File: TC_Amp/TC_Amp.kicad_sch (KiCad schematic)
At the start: 60 parts, among them J1 Screw_Terminal_01x02, J2 Screw_Terminal_01x02, J3 Conn_01x04_Pin, J4 Screw_Terminal_01x02, J5 Screw_Terminal_01x02, Q1 PMOS, U1 LT1025CN8-PBF, U10 LT1025CN8-PBF, U11 LM741, U12 LTC1049CN8_PBF, U13 LTC1049CN8_PBF, U14 LM317T, U2 LTC1049CN8_PBF, U3 LT1054, U4 LM741, U5 LTC1049CN8_PBF, U6 LT1025CN8-PBF, U7 LM741, U8 LTC1049CN8_PBF, U9 LTC1049CN8_PBF

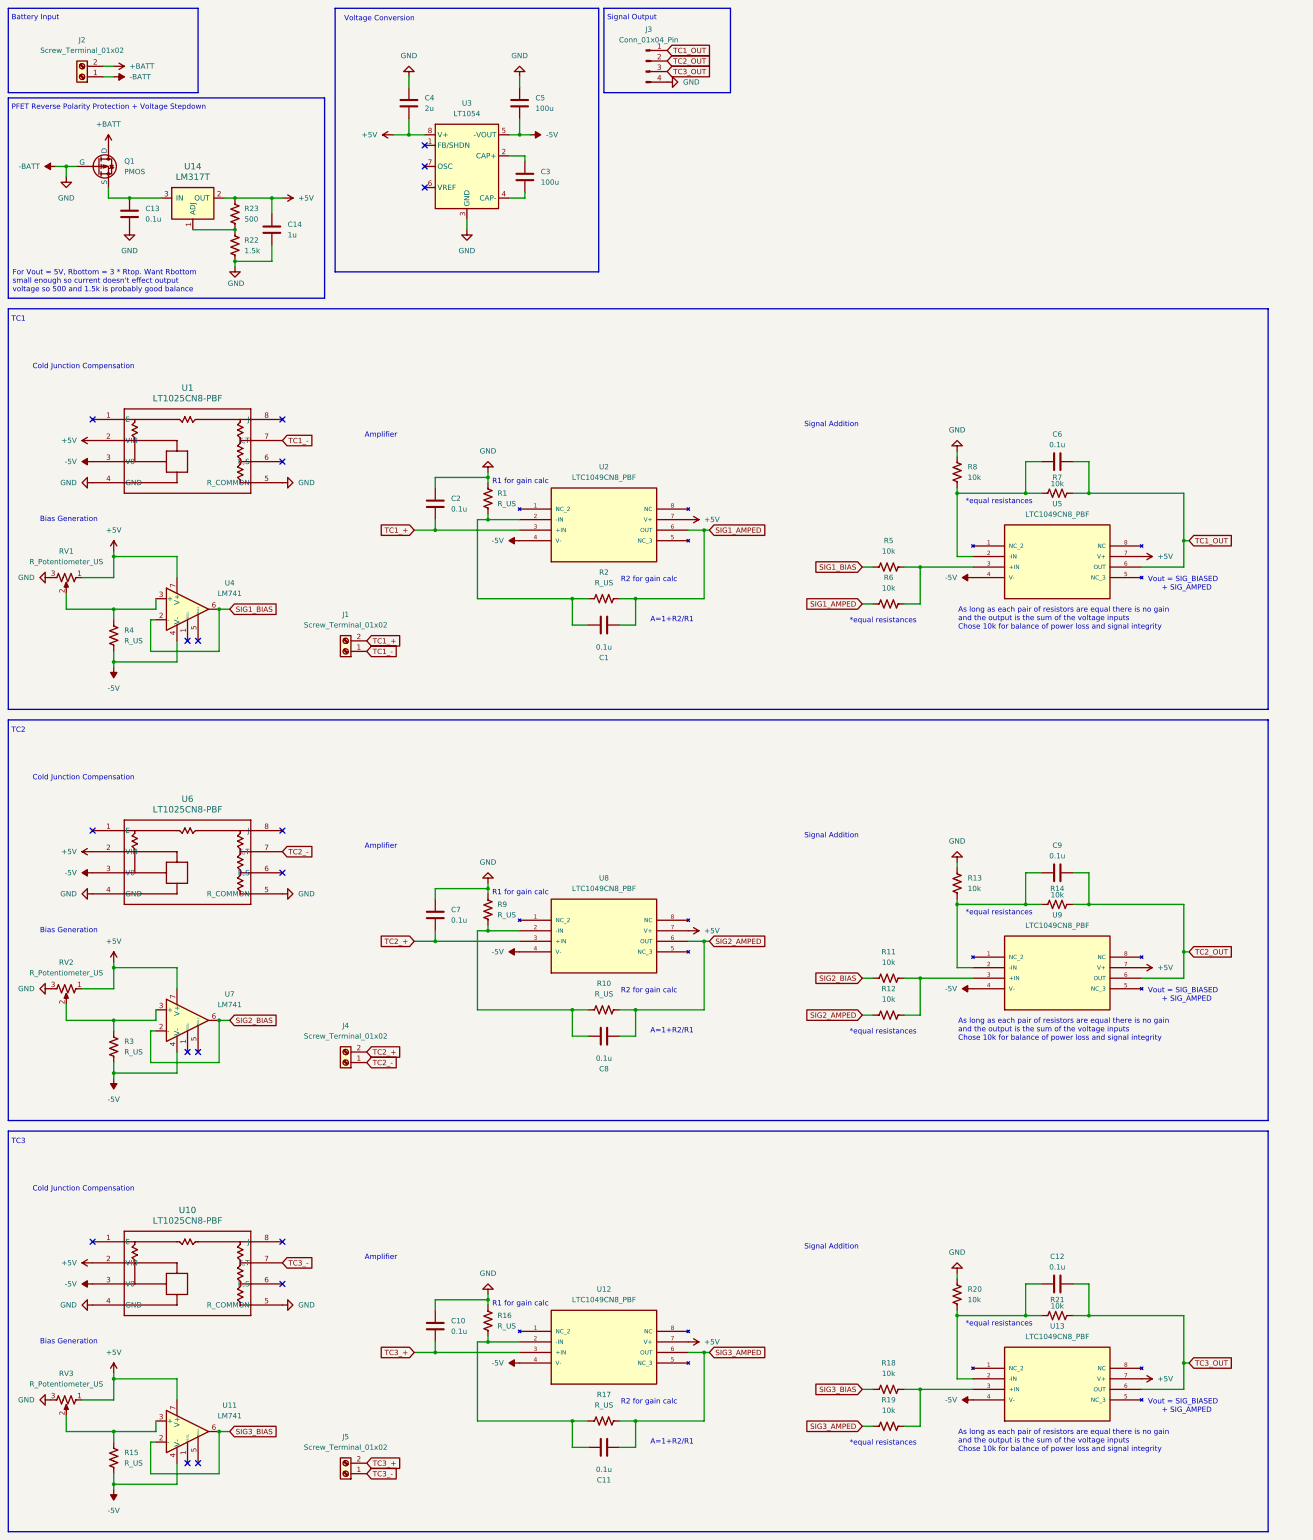
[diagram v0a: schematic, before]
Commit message: change to common cjc
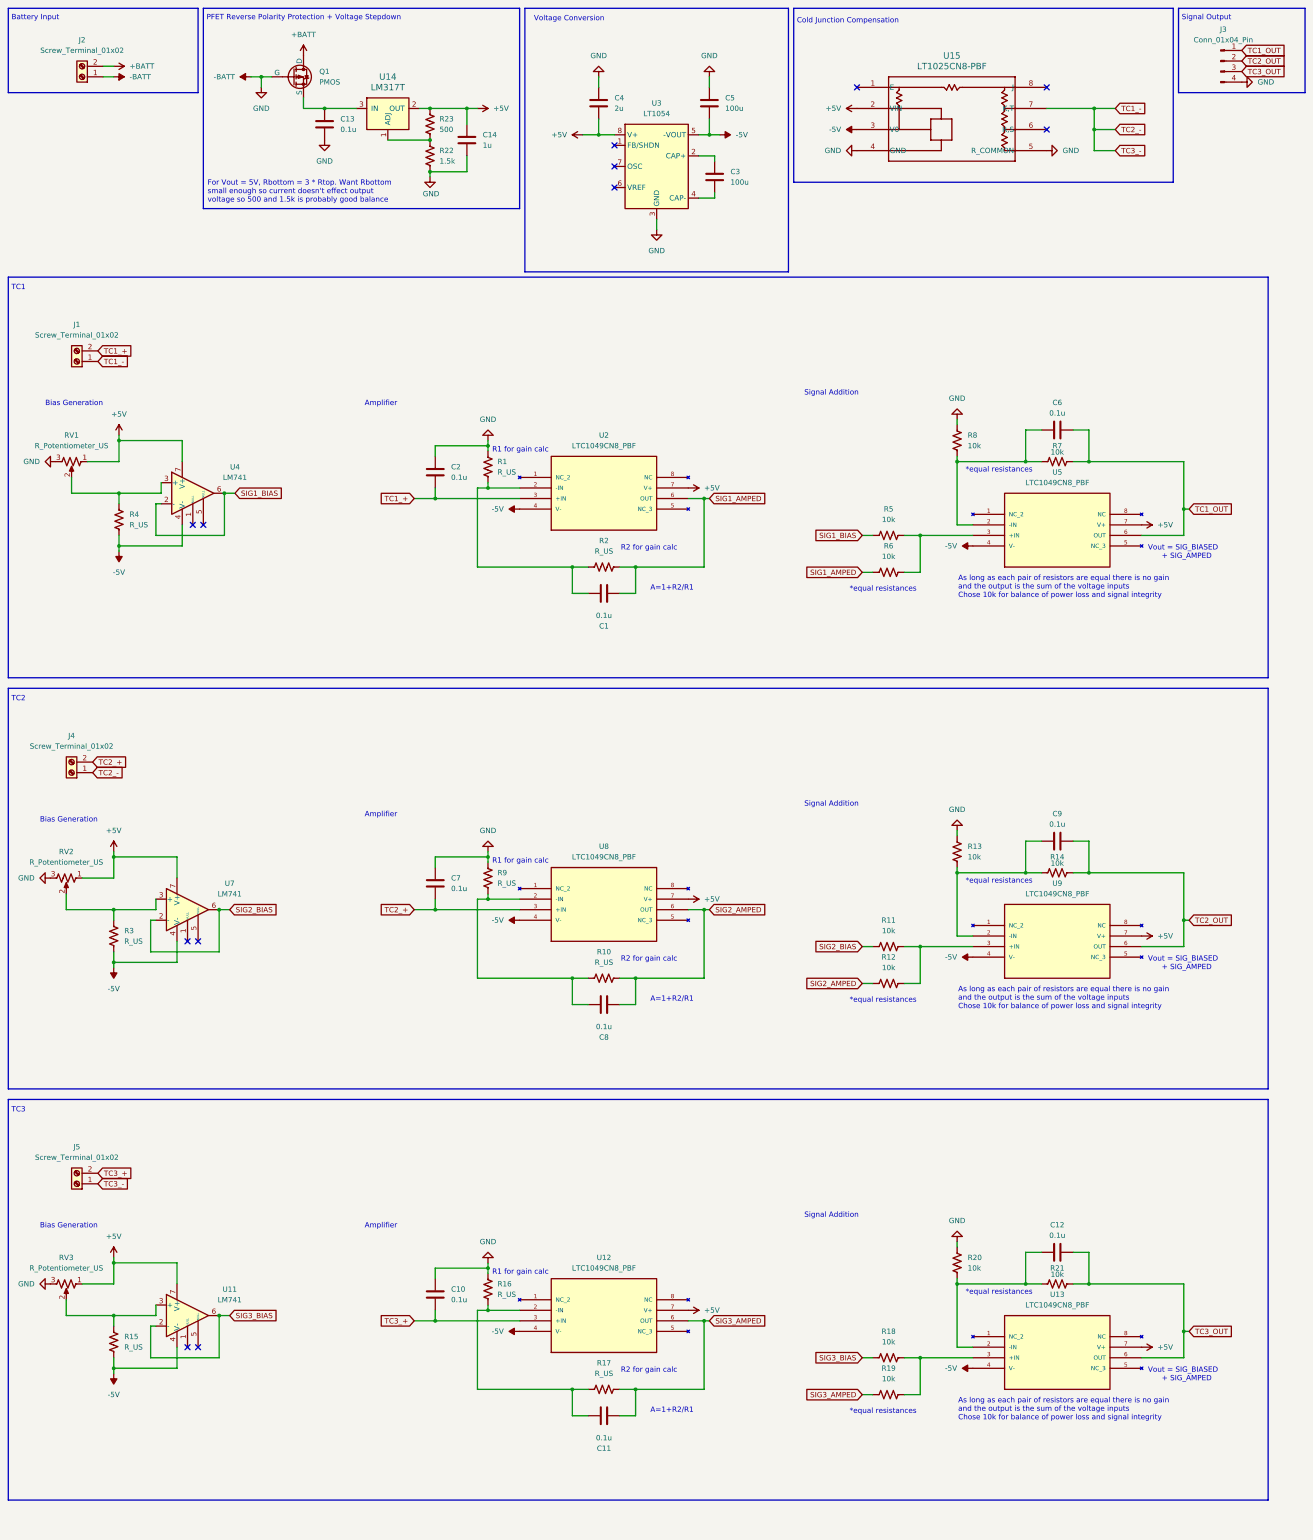
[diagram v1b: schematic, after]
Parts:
- removed U1, U10, U6: LT1025CN8-PBF, Footprints:PDIP8_LT1025CN8-PBF_ADI, symbol 2025-02-03_00-05-09:LT1025CN8-PBF
- added U15: LT1025CN8-PBF, Footprints:PDIP8_LT1025CN8-PBF_ADI, symbol 2025-02-03_00-05-09:LT1025CN8-PBF
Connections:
- net TC2_- is gone; now on net TC1_-: J4.1 (Pin_1)
- net TC3_- is gone; now on net TC1_-: J5.1 (Pin_1)
- net +5V: now also U15.2 (VIN)
- net -5V: now also U15.3 (V0)
- net -BATT: now also U15.4 (GND), U15.5 (R_COMMON)
- net TC1_-: now also U15.7 (K,T)
- no-connect marks 18 -> 12
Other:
- moved on the sheet: C1, C10, C11, C12, C13, C14, C2, C3, C4, C5, C6, C7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

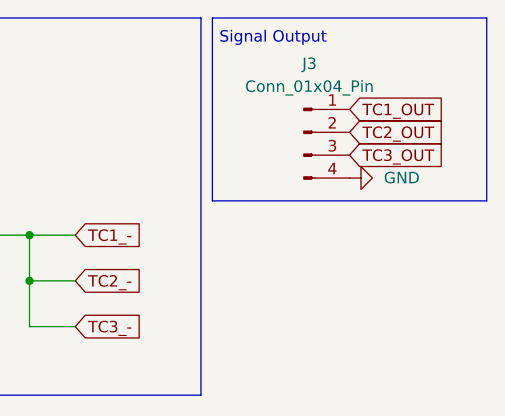
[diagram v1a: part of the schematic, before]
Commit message: finished prelim traces
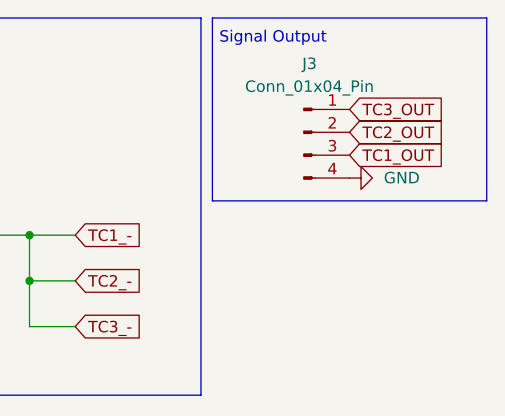
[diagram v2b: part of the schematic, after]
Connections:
- net TC1_OUT: now also J3.3 (Pin_3); no longer J3.1 (Pin_1)
- net TC3_OUT: now also J3.1 (Pin_1); no longer J3.3 (Pin_3)
